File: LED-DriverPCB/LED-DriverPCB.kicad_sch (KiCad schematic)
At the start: 51 parts, among them J1 Screw_Terminal_01x03, J12 Screw_Terminal_01x02, J13 Screw_Terminal_01x02, J14 Screw_Terminal_01x02, J15 Screw_Terminal_01x02, J16 Screw_Terminal_01x02, J17 Screw_Terminal_01x02, J18 Screw_Terminal_01x02, J19 Screw_Terminal_01x02, J2 Screw_Terminal_01x03, J20 Conn_ARM_SWD_TagConnect_TC2030, J3 Screw_Terminal_01x03, J4 Screw_Terminal_01x03, J5 Screw_Terminal_01x03, J6 Screw_Terminal_01x03, J7 Screw_Terminal_01x03, J8 Screw_Terminal_01x03, J9 USB_C_Receptacle_USB2.0_16P, U1 STM32F103RCTx, U2 TXB0108PW, U3 AMS1117-3.3, U4 USBLC6-2SC6, X1 8MHz

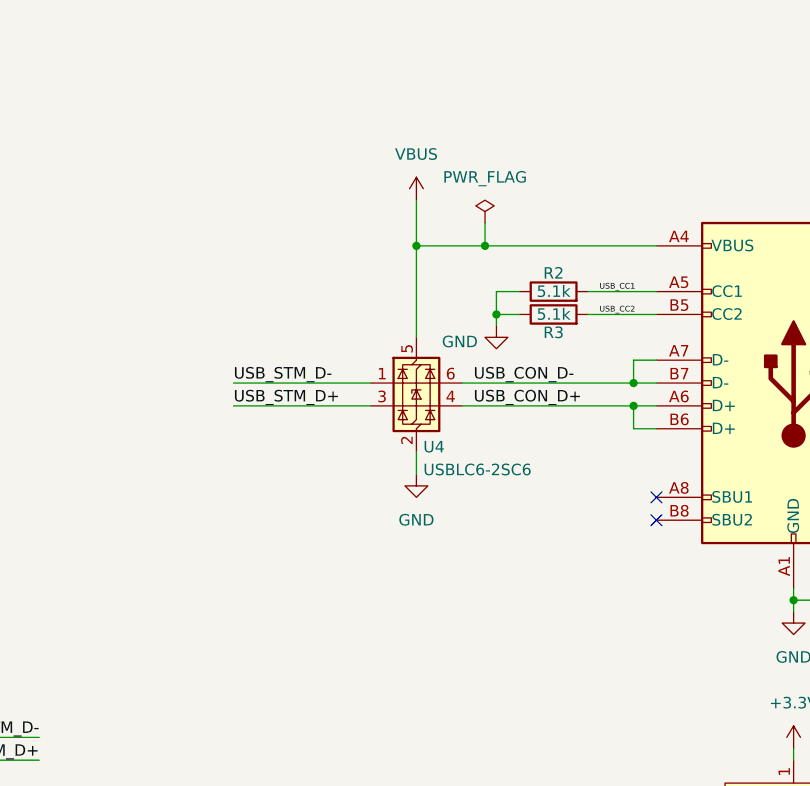
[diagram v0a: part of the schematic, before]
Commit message: Started routing
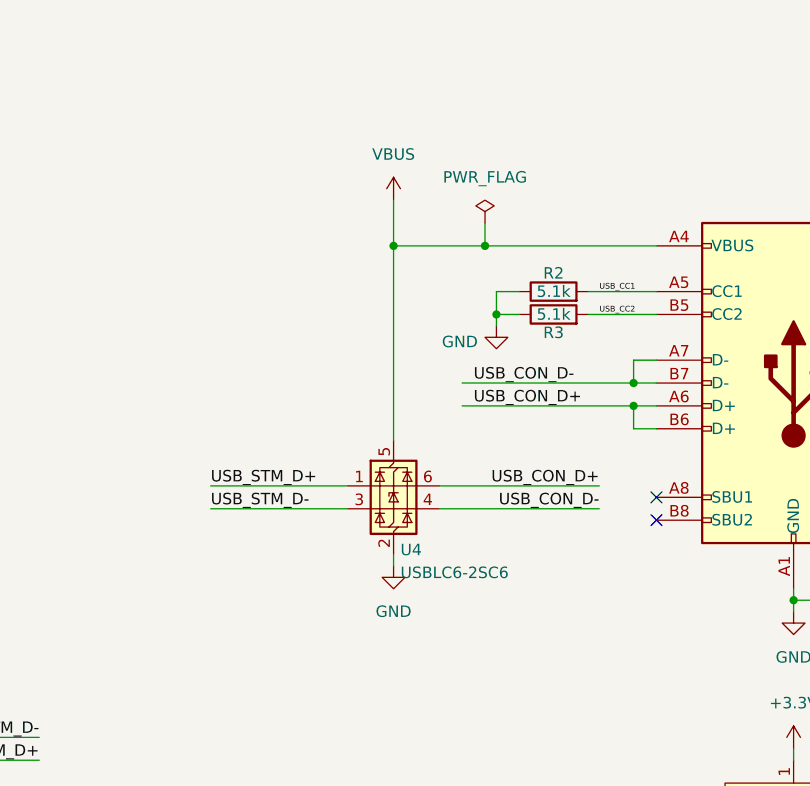
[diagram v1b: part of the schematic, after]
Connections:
- net USB_CON_D+: now also U4.6 (I/O1); no longer U4.4 (I/O2)
- net USB_CON_D-: now also U4.4 (I/O2); no longer U4.6 (I/O1)
- net USB_STM_D+: now also U4.1 (I/O1); no longer U4.3 (I/O2)
- net USB_STM_D-: now also U4.3 (I/O2); no longer U4.1 (I/O1)
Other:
- moved on the sheet: U4
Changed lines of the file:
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@@
 	)
 	(junction
-		(at 191.77 43.18)
-		(diameter 0)
-		(color 0 0 0 0)
-	)
-	(junction
 		(at 78.74 59.69)
 		(diameter 0)
@@
 	)
 	(junction
+		(at 189.23 43.18)
+		(diameter 0)
+		(color 0 0 0 0)
+	)
+	(junction
 		(at 215.9 60.96)
 		(diameter 0)
@@
 	(wire
 		(pts
-			(xy 191.77 43.18) (xy 199.39 43.18)
-		)
-		(stroke
-			(width 0)
-			(type default)
-		)
-	)
-	(wire
-		(pts
 			(xy 66.04 247.65) (xy 80.01 247.65)
 		)
@@
 	(wire
 		(pts
+			(xy 189.23 77.47) (xy 189.23 78.74)
+		)
+		(stroke
+			(width 0)
+			(type default)
+		)
+	)
+	(wire
+		(pts
 			(xy 78.74 45.72) (xy 90.17 45.72)
 		)
@@
 	(wire
 		(pts
-			(xy 171.45 58.42) (xy 186.69 58.42)
+			(xy 168.91 72.39) (xy 184.15 72.39)
 		)
 		(stroke
@@
 	(wire
 		(pts
-			(xy 191.77 66.04) (xy 191.77 68.58)
-		)
-		(stroke
-			(width 0)
-			(type default)
-		)
-	)
-	(wire
-		(pts
 			(xy 210.82 210.82) (xy 223.52 210.82)
 		)
@@
 	(wire
 		(pts
-			(xy 191.77 38.1) (xy 191.77 43.18)
+			(xy 189.23 38.1) (xy 189.23 43.18)
 		)
 		(stroke
@@
 	(wire
 		(pts
-			(xy 171.45 60.96) (xy 186.69 60.96)
+			(xy 168.91 69.85) (xy 184.15 69.85)
 		)
 		(stroke
@@
 	(wire
 		(pts
+			(xy 189.23 43.18) (xy 189.23 64.77)
+		)
+		(stroke
+			(width 0)
+			(type default)
+		)
+	)
+	(wire
+		(pts
 			(xy 66.04 252.73) (xy 80.01 252.73)
 		)
@@
 	(wire
 		(pts
+			(xy 189.23 43.18) (xy 199.39 43.18)
+		)
+		(stroke
+			(width 0)
+			(type default)
+		)
+	)
+	(wire
+		(pts
 			(xy 90.17 45.72) (xy 90.17 49.53)
 		)
@@
 	(wire
 		(pts
+			(xy 194.31 72.39) (xy 212.09 72.39)
+		)
+		(stroke
+			(width 0)
+			(type default)
+		)
+	)
+	(wire
+		(pts
 			(xy 111.76 60.96) (xy 111.76 62.23)
 		)
@@
 	(wire
 		(pts
-			(xy 191.77 43.18) (xy 191.77 53.34)
-		)
-		(stroke
-			(width 0)
-			(type default)
-		)
-	)
-	(wire
-		(pts
 			(xy 67.31 59.69) (xy 78.74 59.69)
 		)
@@
 	(wire
 		(pts
+			(xy 194.31 69.85) (xy 212.09 69.85)
+		)
+		(stroke
+			(width 0)
+			(type default)
+		)
+	)
+	(wire
+		(pts
 			(xy 212.09 115.57) (xy 223.52 115.57)
 		)
@@
 		)
 	)
+	(label "USB_CON_D-"
+		(at 212.09 72.39 180)
+		(effects
+			(font
+				(size 1.27 1.27)
+			)
+			(justify right bottom)
+		)
+	)
 	(label "PWM_TIM5_CH2"
 		(at 29.21 245.11 0)
@@
 		)
 	)
+	(label "USB_CON_D+"
+		(at 212.09 69.85 180)
+		(effects
+			(font
+				(size 1.27 1.27)
+			)
+			(justify right bottom)
+		)
+	)
 	(label "USB_STM_D-"
 		(at 149.86 97.79 180)
@@
 	)
 	(label "USB_STM_D-"
-		(at 171.45 58.42 0)
+		(at 168.91 72.39 0)
 		(effects
 			(font
@@
 	)
 	(label "USB_STM_D+"
-		(at 171.45 60.96 0)
+		(at 168.91 69.85 0)
 		(effects
 			(font
@@
 	(symbol
 		(lib_id "power:GND")
-		(at 191.77 68.58 0)
-		(unit 1)
-		(exclude_from_sim no)
-		(in_bom yes)
-		(on_board yes)
-		(dnp no)
-		(fields_autoplaced yes)
-		(property "Reference" "#PWR09"
-			(at 191.77 74.93 0)
-			(effects
-				(font
-					(size 1.27 1.27)
-				)
-				(hide yes)
-			)
-		)
-		(property "Value" "GND"
-			(at 191.77 73.66 0)
-			(effects
-				(font
-					(size 1.27 1.27)
-				)
-			)
-		)
-		(property "Footprint" ""
-			(at 191.77 68.58 0)
-			(effects
-				(font
-					(size 1.27 1.27)
-				)
-				(hide yes)
-			)
-		)
-		(property "Datasheet" ""
-			(at 191.77 68.58 0)
-			(effects
-				(font
-					(size 1.27 1.27)
-				)
-				(hide yes)
-			)
-		)
-		(property "Description" "Power symbol creates a global label with name \"GND\" , ground"
-			(at 191.77 68.58 0)
-			(effects
-				(font
-					(size 1.27 1.27)
-				)
-				(hide yes)
-			)
-		)
-		(pin "1"
-		)
-		(instances
-			(project "LED-DriverPCB"
-				(path "/f8915909-606a-4747-b712-208c2aaca226"
-					(reference "#PWR09")
-					(unit 1)
-				)
-			)
-		)
-	)
-	(symbol
-		(lib_id "power:GND")
 		(at 21.59 60.96 0)
 		(unit 1)
@@
 	(symbol
 		(lib_id "Power_Protection:USBLC6-2SC6")
-		(at 191.77 58.42 0)
+		(at 189.23 69.85 0)
 		(unit 1)
 		(exclude_from_sim no)
@@
 		(dnp no)
 		(property "Reference" "U4"
-			(at 192.532 65.532 0)
+			(at 189.992 76.962 0)
 			(effects
 				(font
@@
 		)
 		(property "Value" "USBLC6-2SC6"
-			(at 192.532 68.072 0)
+			(at 189.992 79.502 0)
 			(effects
 				(font
@@
 		)
 		(property "Footprint" "Package_TO_SOT_SMD:SOT-23-6"
-			(at 193.04 64.77 0)
+			(at 190.5 76.2 0)
 			(effects
 				(font
@@
 		)
 		(property "Datasheet" "https://www.st.com/resource/en/datasheet/usblc6-2.pdf"
-			(at 193.04 66.675 0)
+			(at 190.5 78.105 0)
 			(effects
 				(font
@@
 		)
 		(property "Description" "Very low capacitance ESD protection diode, 2 data-line, SOT-23-6"
-			(at 191.77 58.42 0)
+			(at 189.23 69.85 0)
 			(effects
 				(font
@@
 	)
 	(symbol
+		(lib_id "power:GND")
+		(at 189.23 78.74 0)
+		(unit 1)
+		(exclude_from_sim no)
+		(in_bom yes)
+		(on_board yes)
+		(dnp no)
+		(fields_autoplaced yes)
+		(property "Reference" "#PWR03"
+			(at 189.23 85.09 0)
+			(effects
+				(font
+					(size 1.27 1.27)
+				)
+				(hide yes)
+			)
+		)
+		(property "Value" "GND"
+			(at 189.23 83.82 0)
+			(effects
+				(font
+					(size 1.27 1.27)
+				)
+			)
+		)
+		(property "Footprint" ""
+			(at 189.23 78.74 0)
+			(effects
+				(font
+					(size 1.27 1.27)
+				)
+				(hide yes)
+			)
+		)
+		(property "Datasheet" ""
+			(at 189.23 78.74 0)
+			(effects
+				(font
+					(size 1.27 1.27)
+				)
+				(hide yes)
+			)
+		)
+		(property "Description" "Power symbol creates a global label with name \"GND\" , ground"
+			(at 189.23 78.74 0)
+			(effects
+				(font
+					(size 1.27 1.27)
+				)
+				(hide yes)
+			)
+		)
+		(pin "1"
+		)
+		(instances
+			(project ""
+				(path "/f8915909-606a-4747-b712-208c2aaca226"
+					(reference "#PWR03")
+					(unit 1)
+				)
+			)
+		)
+	)
+	(symbol
 		(lib_id "Connector:Screw_Terminal_01x03")
 		(at 228.6 213.36 0)
@@
 	(symbol
 		(lib_id "power:VBUS")
-		(at 191.77 38.1 0)
+		(at 189.23 38.1 0)
 		(unit 1)
 		(exclude_from_sim no)
@@
 		(fields_autoplaced yes)
 		(property "Reference" "#PWR08"
-			(at 191.77 41.91 0)
+			(at 189.23 41.91 0)
 			(effects
 				(font
@@
 		)
 		(property "Value" "VBUS"
-			(at 191.77 33.02 0)
+			(at 189.23 33.02 0)
 			(effects
 				(font
@@
 		)
 		(property "Footprint" ""
-			(at 191.77 38.1 0)
+			(at 189.23 38.1 0)
 			(effects
 				(font
@@
 		)
 		(property "Datasheet" ""
-			(at 191.77 38.1 0)
+			(at 189.23 38.1 0)
 			(effects
 				(font
@@
 		)
 		(property "Description" "Power symbol creates a global label with name \"VBUS\""
-			(at 191.77 38.1 0)
+			(at 189.23 38.1 0)
 			(effects
 				(font
